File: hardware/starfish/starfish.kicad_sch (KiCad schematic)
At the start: 4 parts

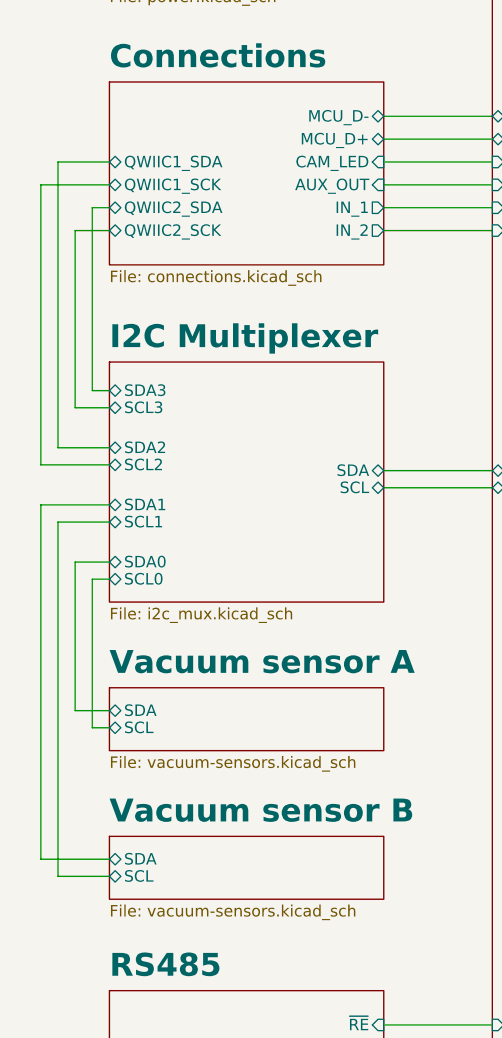
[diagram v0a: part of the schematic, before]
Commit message: First pass at layout and routing
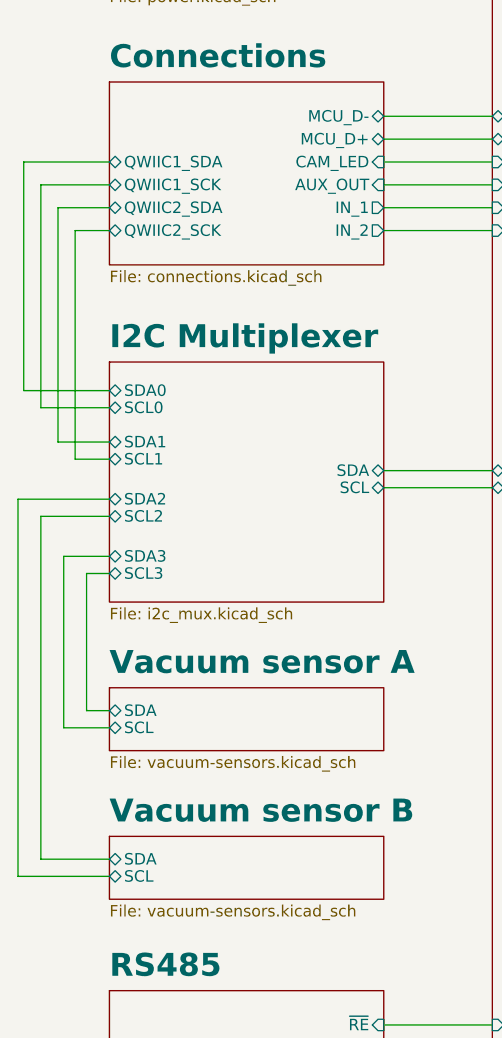
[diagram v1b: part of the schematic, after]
